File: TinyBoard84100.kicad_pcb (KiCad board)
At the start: 2 copper layers, 14 parts, among them P1 CONN_01X02, P2 CONN_01X07, P3 CONN_01X07, P4 CONN_02X03, SW1 SW_PUSH, U1 78L05, U2 ATTINY841

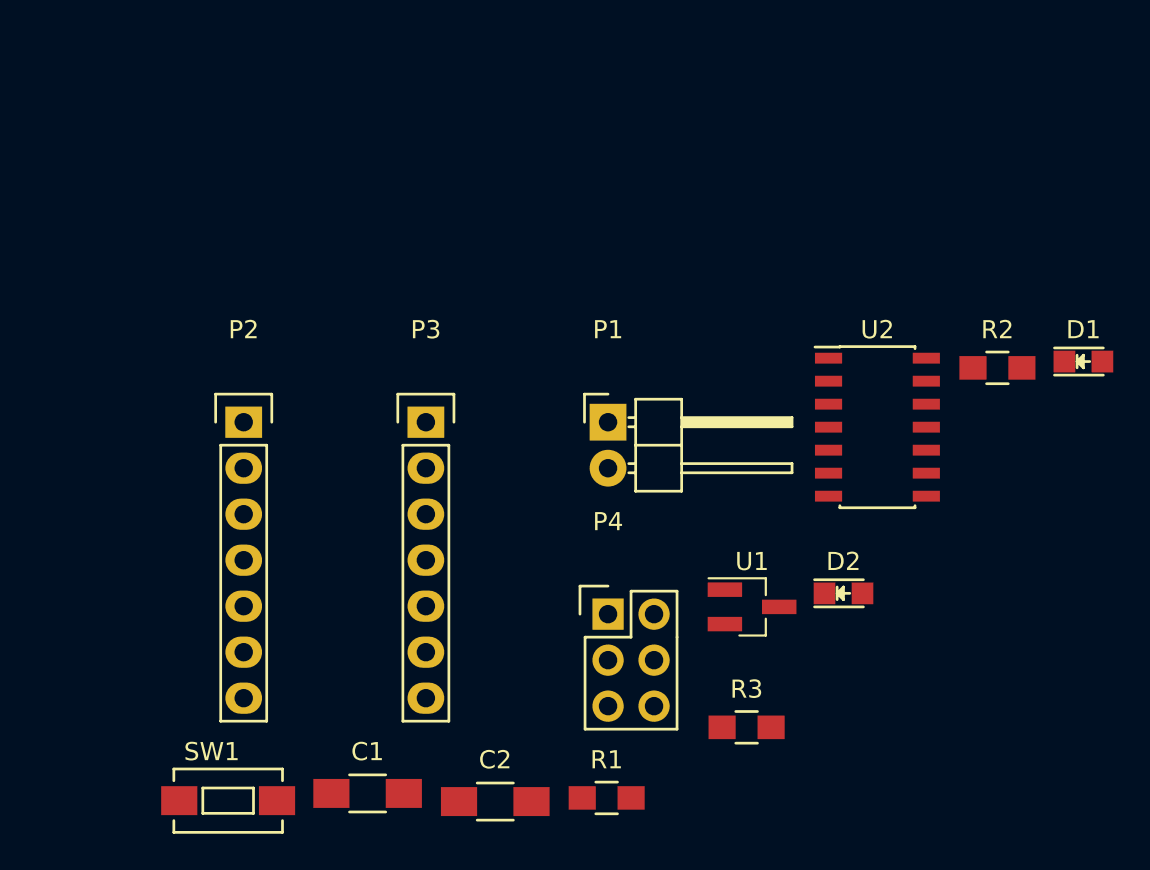
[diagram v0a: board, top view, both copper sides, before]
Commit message: First layout
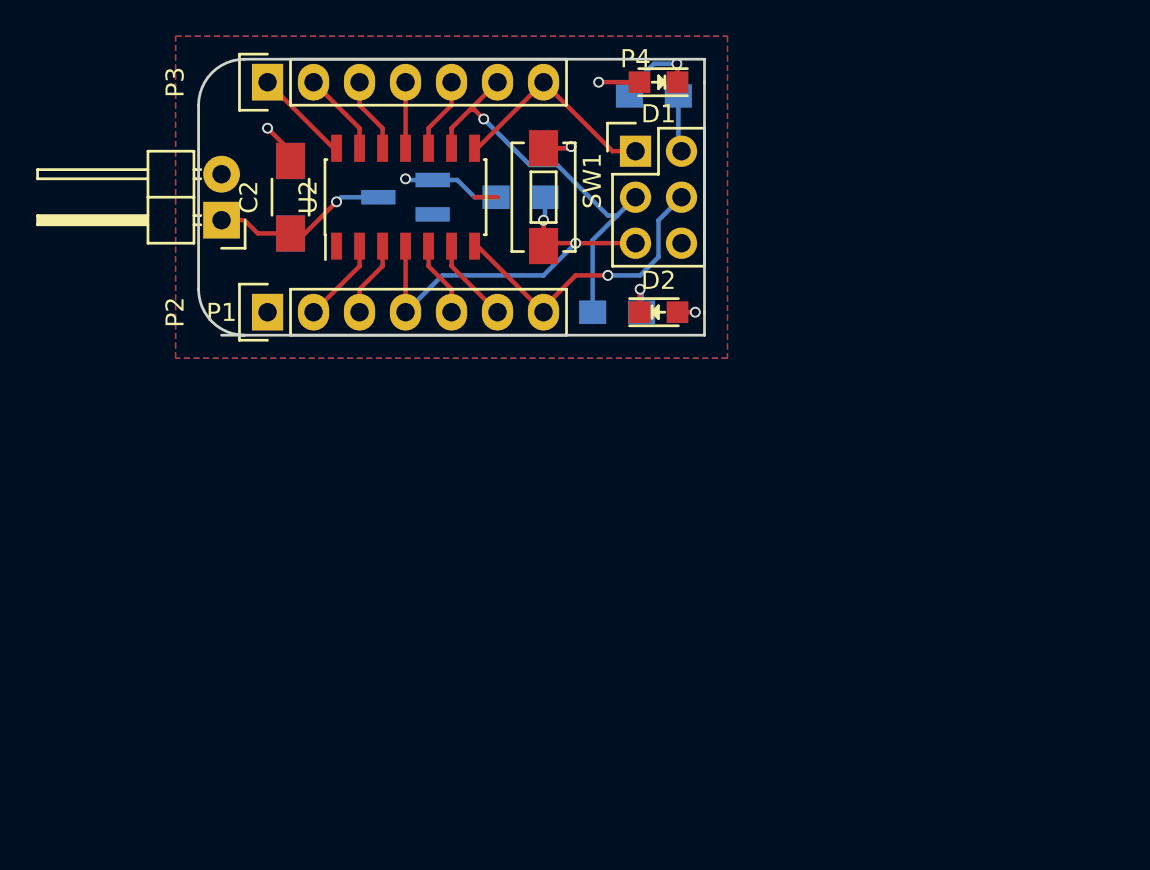
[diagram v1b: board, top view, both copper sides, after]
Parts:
- C1, R1, R2, R3, U1: moved to B.Cu
- moved SW1 37.6 mm to (172.7, 80.0), turned to 270 degrees
- moved C2 35.2 mm to (158.8, 80.0), turned to 90 degrees
- moved R1 33.5 mm to (171.4, 80.0)
- moved C1 33.2 mm to (158.8, 80.0), turned to 90 degrees
- moved U1 29.6 mm to (165.1, 80.0), turned to 180 degrees
- moved U2 29.0 mm to (165.1, 80.0), turned to 90 degrees
- moved D1 28.1 mm to (179.1, 73.7), turned to 180 degrees
- moved P4 25.6 mm to (177.8, 77.5)
- moved R2 24.2 mm to (178.8, 74.4), turned to 180 degrees
- moved P1 24.1 mm to (154.9, 81.3), turned to 180 degrees
- moved R3 24.0 mm to (176.8, 86.4)
- moved P3 20.7 mm to (157.5, 73.7), turned to 90 degrees
- moved D2 18.6 mm to (179.1, 86.4)
- moved P2 6.22 mm to (157.5, 86.4), turned to 90 degrees
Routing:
- net /PA4: track 0.00 -> 22.6 mm, vias 0 -> 1
- net /PB3: track 0.00 -> 22.5 mm, vias 0 -> 2
- net /PA6: track 0.00 -> 16.9 mm, vias 0 -> 1
- net GND: track 0.00 -> 13.4 mm, vias 0 -> 4
- net /PA5: track 0.00 -> 12.0 mm
- net Net-(C1-Pad1): track 0.00 -> 9.79 mm, vias 0 -> 1
- net +5V: track 0.00 -> 8.70 mm, vias 0 -> 1
- net /PA7: track 0.00 -> 4.70 mm
- net /PB0: track 0.00 -> 4.70 mm
- net /PA0: track 0.00 -> 4.70 mm
- net Net-(D1-Pad1): track 0.00 -> 4.64 mm, vias 0 -> 1
- net /PA1: track 0.00 -> 4.18 mm
- net /PB1: track 0.00 -> 4.18 mm
- net /PA3: track 0.00 -> 4.18 mm
- net /PB2: track 0.00 -> 4.18 mm
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- added copper zone on F.Cu, net +5V
- added copper zone on B.Cu, net GND
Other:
- board outline added: 27.9 x 15.2 mm
